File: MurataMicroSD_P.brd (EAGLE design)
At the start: 80 x 76 mm, 91 parts, among them CON1 CON_TC2030-CTL-NL, CON2 CON_TC2030-CTL-NL, CON3 CON_TC2030-CTL-NL, CON4 CON_TC2030-CTL-NL, CON5 CON_TC2030-CTL-NL, CON6 CON_TC2030-CTL-NL, CON7 CON_TC2030-CTL-NL, CON8 CON_TC2030-CTL-NL, U1 IC_BLE_LBCA2HNZYZ-711, U2 IC_BLE_LBCA2HNZYZ-711, U3 IC_BLE_LBCA2HNZYZ-711, U4 IC_BLE_LBCA2HNZYZ-711, U5 IC_BLE_LBCA2HNZYZ-711, U6 IC_BLE_LBCA2HNZYZ-711, U7 IC_BLE_LBCA2HNZYZ-711, U8 IC_BLE_LBCA2HNZYZ-711

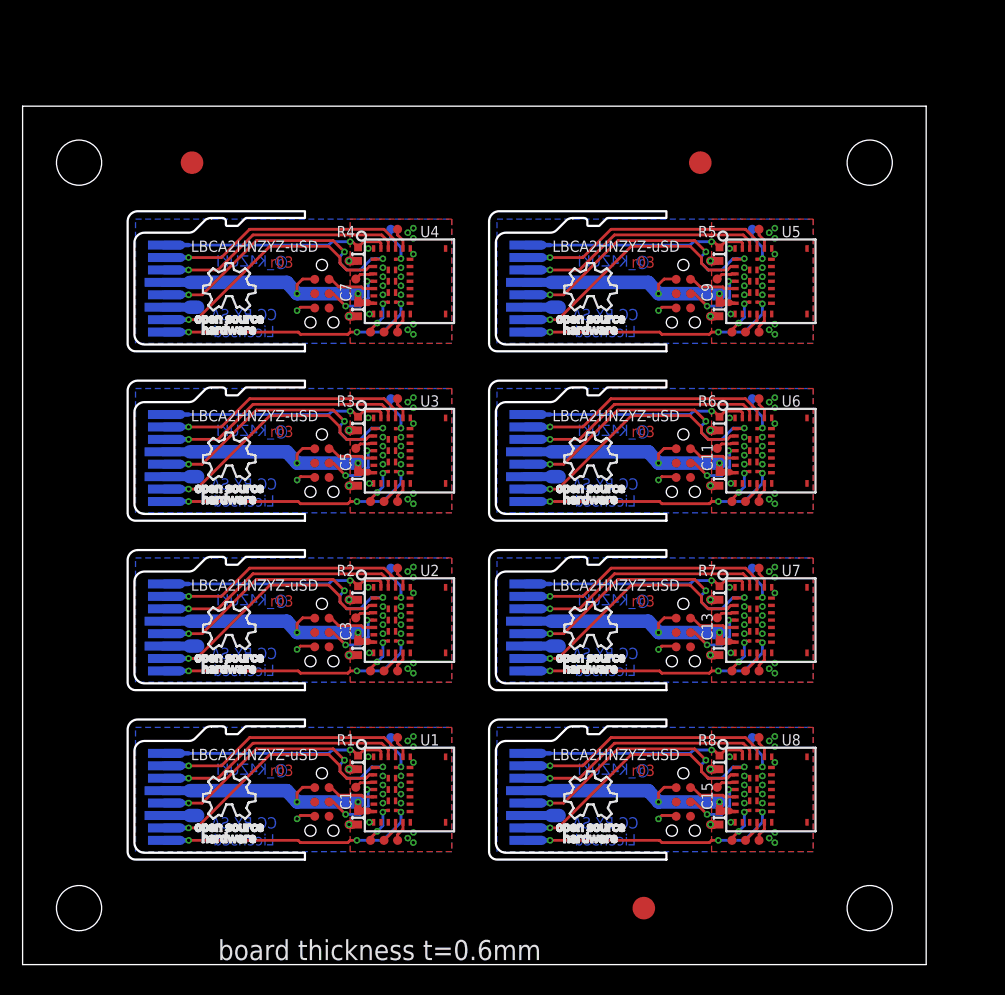
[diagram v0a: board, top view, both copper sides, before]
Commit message: [ uSD ] panelised as r3
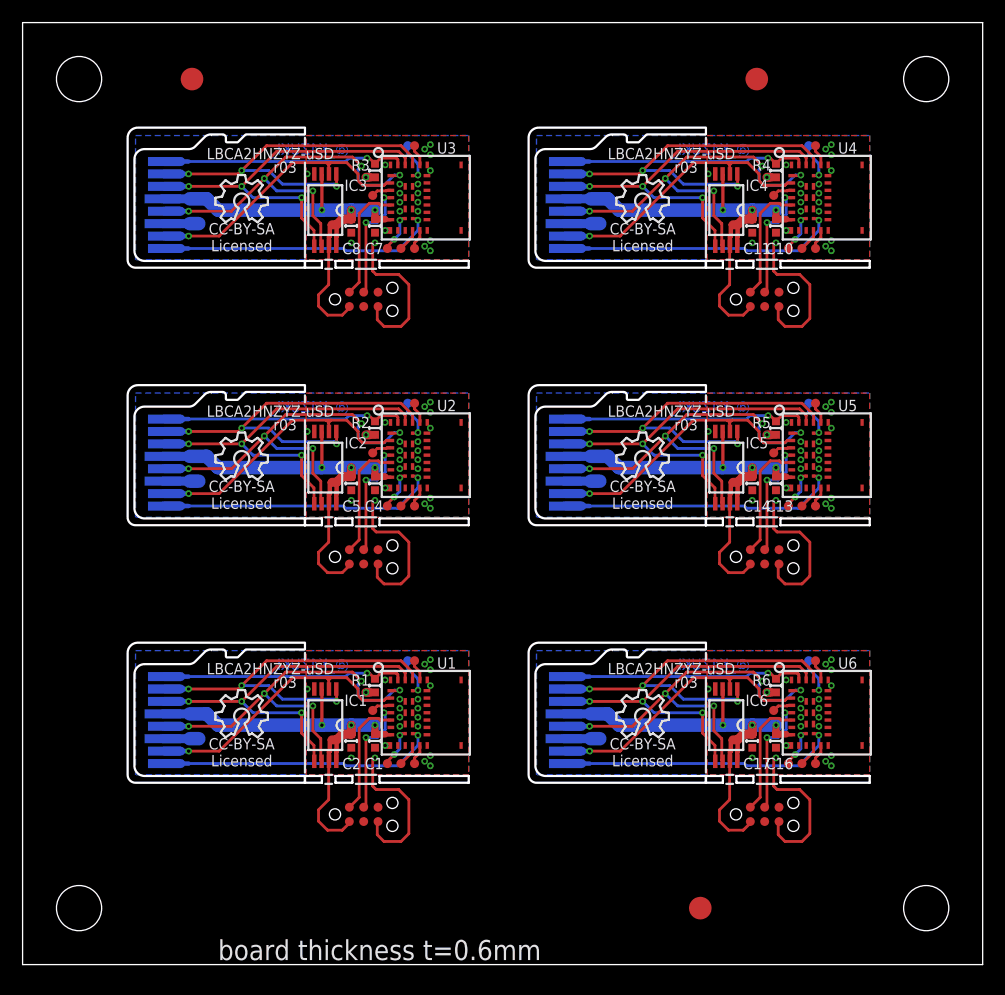
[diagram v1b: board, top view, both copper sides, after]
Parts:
- removed CON7, CON8: CON_TC2030-CTL-NL, mylib:CON_TC2030-IDC-NL
- removed R7, R8: (no value), mylib:C0402
- removed TP37, TP38, TP39, TP40, TP41, TP42, TP43, TP44, TP45, TP46, TP47, TP48, TP49, TP50, TP51: TPTP08R, testpad_local:TP08R
- removed U7, U8: IC_BLE_LBCA2HNZYZ-711, mylib:IC_MURATA_LBCA2HNZYZ-711
- added C16, C17: (no value), mylib:C0402
- added IC1, IC2, IC3, IC4, IC5, IC6: 1265-1139-1-ND, mylib:IC_08_0.65_160MIL
- added TP100, TP101, TP102: TPTP20R, testpad_local:TP20R
- added U$1, U$2, U$3, U$4, U$5, U$6: ICON_OSHW, mylib:ICON_OSHW
- C10, C14, C2, C4, C8: value BOARD_MICROSD -> (none); device mylib:BOARD_MICROSD -> mylib:C0402
- C15, C3, C9: value (none) -> BOARD_MICROSD; device mylib:C0402 -> mylib:BOARD_MICROSD
- TP3, TP4, TP5: value TPTP20R -> TPTP08R; device testpad_local:TP20R -> testpad_local:TP08R
- moved TP4 49.1 mm to (34.7, 49.7)
- moved TP21 48.7 mm to (70.2, 72.5)
- moved TP31 47.5 mm to (69.0, 17.8), flipped to the top
- moved TP20 45.3 mm to (70.2, 63.4)
- moved TP25 43.9 mm to (69.0, 40.6), flipped to the top
- moved TP26 42.3 mm to (70.2, 40.6)
- moved TP27 42.2 mm to (70.2, 49.7)
- moved TP15 42.1 mm to (34.7, 72.5)
- moved TP22 41.1 mm to (69.6, 72.5), flipped to the bottom
- moved CON4 39.2 mm to (65.7, 58.9), turned to 0 degrees
- moved TP32 38.9 mm to (70.2, 17.8)
- moved TP19 38.8 mm to (69.0, 63.4), flipped to the top
- moved R4 37.7 mm to (66.7, 70.3)
- moved U4 37.7 mm to (67.5, 71.4)
- moved TP14 37.6 mm to (34.7, 63.4)
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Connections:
- net N$2 renamed VPP
- removed net !CS!6: C12.2_CS, U7.23
- removed net !CS!7: C14.2_CS, U8.23
- removed net 3.3V6: C12.4_VDD, C13.1, CON7.1, U7.7
- removed net 3.3V7: C14.4_VDD, C15.1, CON8.1, U8.7
- removed net DAT1: TP1.TP, U1.3
- removed net DAT2: TP15.TP, U2.3
- removed net DAT3: TP21.TP, U3.3
- removed net DAT4: TP27.TP, U4.3
- removed net DAT5: TP33.TP, U5.3
- removed net DAT6: TP39.TP, U6.3
- removed net DAT7: TP45.TP, U7.3
- removed net DAT8: TP51.TP, U8.3
- removed net GND6: C12.6_VSS, C13.2, CON7.5, R7.1, U7.15, U7.16, U7.17, U7.18, U7.20, U7.21, U7.26, U7.27, U7.28, U7.29, U7.32, U7.33, U7.34, U7.6, U7.8
- removed net GND7: C14.6_VSS, C15.2, CON8.5, R8.1, U8.15, U8.16, U8.17, U8.18, U8.20, U8.21, U8.26, U8.27, U8.28, U8.29, U8.32, U8.33, U8.34, U8.6, U8.8
- removed net MISO6: C12.7_MISO, U7.2
- removed net MISO7: C14.7_MISO, U8.2
- removed net N$10: C8.8_DAT1, U5.31
- removed net N$11: C10.1_DAT2, R6.2, U6.25
- removed net N$12: C10.8_DAT1, U6.31
- removed net N$13: C12.1_DAT2, R7.2, U7.25
- removed net N$14: C12.8_DAT1, U7.31
- removed net N$15: C14.1_DAT2, R8.2, U8.25
- removed net N$16: C14.8_DAT1, U8.31
- removed net N$7: C6.1_DAT2, R4.2, U4.25
- removed net N$8: C6.8_DAT1, U4.31
- removed net N$9: C8.1_DAT2, R5.2, U5.25
- removed net P1_12: TP43.TP, U7.35
- removed net P1_13: TP44.TP, U7.30
- removed net P1_14: TP49.TP, U8.35
- removed net P1_15: TP50.TP, U8.30
- removed net RXD_MOSI6: C12.3_MOSI, U7.24
- removed net RXD_MOSI7: C14.3_MOSI, U8.24
- removed net SCK6: C12.5_CLK, U7.1
- removed net SCK7: C14.5_CLK, U8.1
- removed net SWCLK6: CON7.4, U7.4
- removed net SWCLK7: CON8.4, U8.4
- removed net SWDIO6: CON7.2, U7.5
- removed net SWDIO7: CON8.2, U8.5
- new net N$2: C3.1_DAT2, R2.2, U2.25
- new net VPP1: C3.8_DAT1, U2.31
- new net VPP2: C6.8_DAT1, U3.31
- new net VPP3: C9.8_DAT1, U4.31
- new net VPP4: C12.8_DAT1, U5.31
- new net VPP5: C15.8_DAT1, U6.31
- net !CS!: now also IC1.1
- net !CS!1: now also C3.2_CS, IC2.1; no longer C2.2_CS
- net !CS!2: now also C6.2_CS, IC3.1; no longer C4.2_CS
- net !CS!3: now also C9.2_CS, IC4.1; no longer C6.2_CS
- net !CS!4: now also C12.2_CS, IC5.1; no longer C8.2_CS
- net !CS!5: now also C15.2_CS, IC6.1; no longer C10.2_CS
- net 3.3V: now also C2.1, IC1.3, IC1.7, IC1.8
- net 3.3V1: now also C3.4_VDD, C4.1, C5.1, IC2.3, IC2.7, IC2.8; no longer C2.4_VDD, C3.1
- net 3.3V2: now also C6.4_VDD, C7.1, C8.1, IC3.3, IC3.7, IC3.8; no longer C4.4_VDD, C5.1
- net 3.3V3: now also C10.1, C11.1, C9.4_VDD, IC4.3, IC4.7, IC4.8; no longer C6.4_VDD, C7.1
- net 3.3V4: now also C12.4_VDD, C13.1, C14.1, IC5.3, IC5.7, IC5.8; no longer C8.4_VDD, C9.1
- net 3.3V5: now also C15.4_VDD, C16.1, C17.1, IC6.3, IC6.7, IC6.8; no longer C10.4_VDD, C11.1
- net GND: now also C2.2, IC1.4
- net GND1: now also C3.6_VSS, C4.2, C5.2, IC2.4; no longer C2.6_VSS, C3.2
- net GND2: now also C6.6_VSS, C7.2, C8.2, IC3.4; no longer C4.6_VSS, C5.2
- net GND3: now also C10.2, C11.2, C9.6_VSS, IC4.4; no longer C6.6_VSS, C7.2
- net GND4: now also C12.6_VSS, C13.2, C14.2, IC5.4; no longer C8.6_VSS, C9.2
- net GND5: now also C15.6_VSS, C16.2, C17.2, IC6.4; no longer C10.6_VSS, C11.2
- net MISO: now also IC1.2
- net MISO1: now also C3.7_MISO, IC2.2; no longer C2.7_MISO
- net MISO2: now also C6.7_MISO, IC3.2; no longer C4.7_MISO
- net MISO3: now also C9.7_MISO, IC4.2; no longer C6.7_MISO
- net MISO4: now also C12.7_MISO, IC5.2; no longer C8.7_MISO
- net MISO5: now also C15.7_MISO, IC6.2; no longer C10.7_MISO
- net N$3: now also C6.1_DAT2, R3.2, U3.25; no longer C2.1_DAT2, R2.2, U2.25
- net N$4: now also C9.1_DAT2, R4.2, U4.25; no longer C2.8_DAT1, U2.31
- net N$5: now also C12.1_DAT2, R5.2, U5.25; no longer C4.1_DAT2, R3.2, U3.25
- net N$6: now also C15.1_DAT2, R6.2, U6.25; no longer C4.8_DAT1, U3.31
- net P0_10: now also TP13.TP, U3.11; no longer TP22.TP, U4.11
- net P0_11: now also TP14.TP, U3.12; no longer TP23.TP, U4.12
- net P0_12: now also TP15.TP, U3.22; no longer TP24.TP, U4.22
- net P0_13: now also TP24.TP, U4.3; no longer TP28.TP, U5.11
- net P0_14: now also TP19.TP, U4.11; no longer TP29.TP, U5.12
- net P0_15: now also TP20.TP, U4.12; no longer TP30.TP, U5.22
- net P0_16: now also TP21.TP, U4.22; no longer TP34.TP, U6.11
- net P0_17: now also TP30.TP, U5.3; no longer TP35.TP, U6.12
- net P0_18: now also TP25.TP, U5.11; no longer TP36.TP, U6.22
- net P0_19: now also TP26.TP, U5.12; no longer TP40.TP, U7.11
- net P0_20: now also TP27.TP, U5.22; no longer TP41.TP, U7.12
- net P0_21: now also TP36.TP, U6.3; no longer TP42.TP, U7.22
- net P0_22: now also TP31.TP, U6.11; no longer TP46.TP, U8.11
- net P0_23: now also TP32.TP, U6.12; no longer TP47.TP, U8.12
- net P0_24: now also TP33.TP, U6.22; no longer TP48.TP, U8.22
- net P0_4: now also TP12.TP, U2.3; no longer TP2.TP, U2.11
- net P0_5: now also TP2.TP, U2.11; no longer TP6.TP, U2.12
- net P0_6: now also TP1.TP, U1.3; no longer TP12.TP, U2.22
- net P0_7: now also TP3.TP, U2.12; no longer TP16.TP, U3.11
- net P0_8: now also TP4.TP, U2.22; no longer TP17.TP, U3.12
- net P0_9: now also U3.3; no longer U3.22
- net P1_10: now also TP34.TP; no longer TP37.TP
- net P1_11: now also TP35.TP; no longer TP38.TP
- net P1_2: now also TP5.TP; no longer TP13.TP
- net P1_3: now also TP6.TP; no longer TP14.TP
- net P1_4: now also TP16.TP; no longer TP19.TP
- net P1_5: now also TP17.TP; no longer TP20.TP
- net P1_6: now also TP22.TP; no longer TP25.TP
- net P1_7: now also TP23.TP; no longer TP26.TP
- net P1_8: now also TP28.TP; no longer TP31.TP
- net P1_9: now also TP29.TP; no longer TP32.TP
- net RXD_MOSI: now also IC1.5
- net RXD_MOSI1: now also C3.3_MOSI, IC2.5; no longer C2.3_MOSI
- net RXD_MOSI2: now also C6.3_MOSI, IC3.5; no longer C4.3_MOSI
- net RXD_MOSI3: now also C9.3_MOSI, IC4.5; no longer C6.3_MOSI
- net RXD_MOSI4: now also C12.3_MOSI, IC5.5; no longer C8.3_MOSI
- net RXD_MOSI5: now also C15.3_MOSI, IC6.5; no longer C10.3_MOSI
- net SCK: now also IC1.6
- net SCK1: now also C3.5_CLK, IC2.6; no longer C2.5_CLK
- net SCK2: now also C6.5_CLK, IC3.6; no longer C4.5_CLK
- net SCK3: now also C9.5_CLK, IC4.6; no longer C6.5_CLK
- net SCK4: now also C12.5_CLK, IC5.6; no longer C8.5_CLK
- net SCK5: now also C15.5_CLK, IC6.6; no longer C10.5_CLK
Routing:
- net SCK6: track 24.8 -> 0.00 mm, vias 3 -> 0
- net SCK7: track 24.8 -> 0.00 mm, vias 3 -> 0
- net VPP4: track 0.00 -> 24.7 mm, vias 0 -> 1
- net VPP1: track 0.00 -> 24.7 mm, vias 0 -> 1
- net VPP5: track 0.00 -> 24.7 mm, vias 0 -> 1
- net VPP2: track 0.00 -> 24.7 mm, vias 0 -> 1
- net VPP3: track 0.00 -> 24.7 mm, vias 0 -> 1
- net N$8: track 23.2 -> 0.00 mm, vias 3 -> 0
- net N$16: track 23.2 -> 0.00 mm, vias 3 -> 0
- net N$14: track 23.2 -> 0.00 mm, vias 3 -> 0
- net N$12: track 23.2 -> 0.00 mm, vias 3 -> 0
- net N$10: track 23.2 -> 0.00 mm, vias 3 -> 0
- net !CS!7: track 22.6 -> 0.00 mm, vias 1 -> 0
- net !CS!6: track 22.6 -> 0.00 mm, vias 1 -> 0
- net 3.3V6: track 22.6 -> 0.00 mm, vias 2 -> 0
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- removed copper zone on layer 1, net GND6
- removed copper zone on layer 16, net GND6
- removed copper zone on layer 1, net GND7
- removed copper zone on layer 16, net GND7
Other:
- board size 80 x 76 mm -> 85 x 83.4 mm
- board text added: "C2"
- board text added: "IC1"
